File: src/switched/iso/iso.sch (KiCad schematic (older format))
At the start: 64 parts, among them IC1 NCP1252ADR2G, J1 Conn_01x02, J2 Conn_01x02, J3 Conn_01x02, J4 Conn_01x02, Q1 TSD5N50MR, Q2 TSD5N50MR, T1 Transformer_1P_1S, U1 NCP5106, U2 ORPC-817C, U3 TL431LP, U4 MC34072, U5 LM317_SOT-223

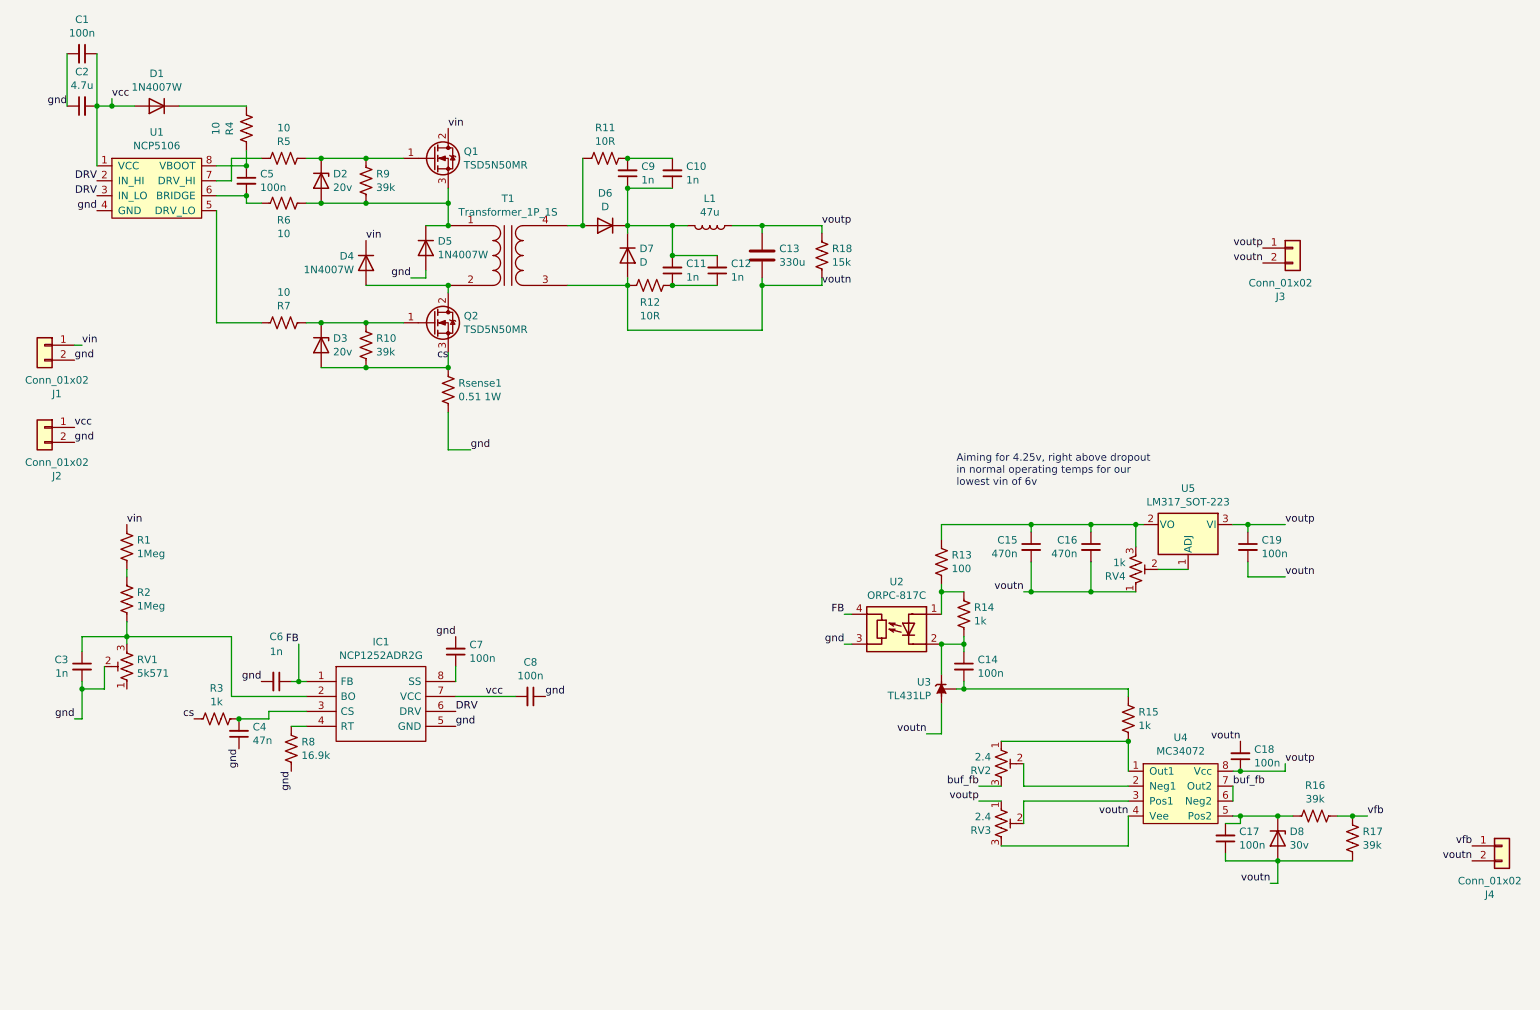
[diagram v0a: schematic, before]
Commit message: Midterm report
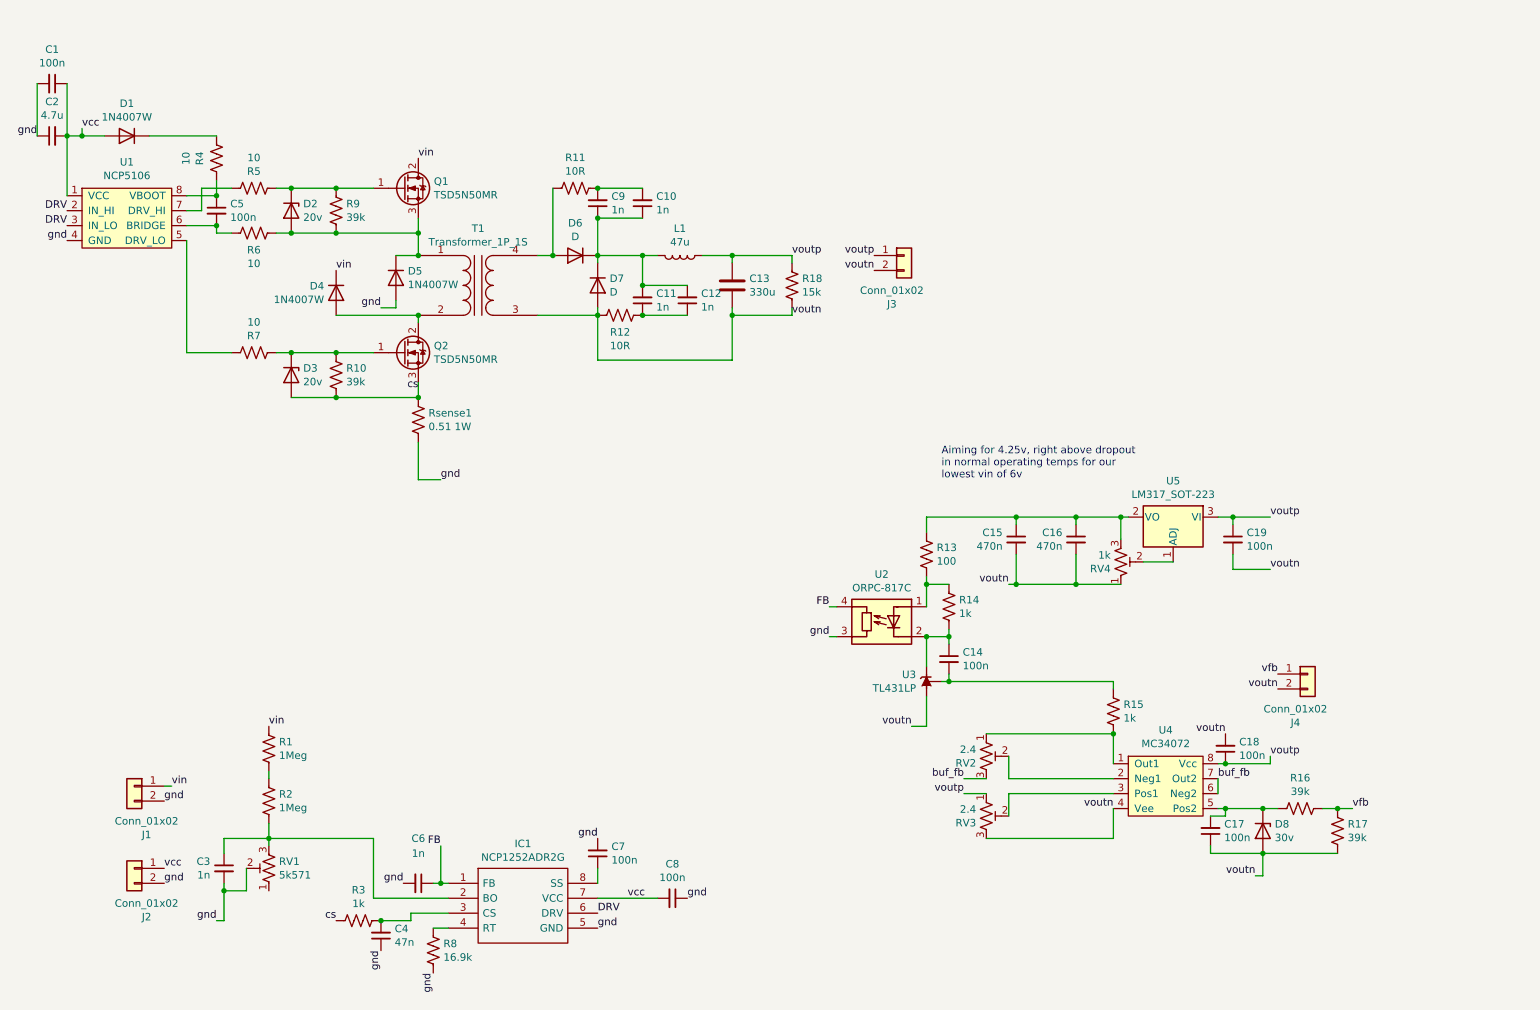
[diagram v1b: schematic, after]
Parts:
- C1, C14, C17, C18, C19, C5, C7, C8: Price (none) -> 0.0032
- C10, C11, C12, C3, C6, C9, R14, R15, R3: Price (none) -> 0.0031
- C13: Price (none) -> 0.1728
- C15, C16: Price (none) -> 0.0112
- C2: Price (none) -> 0.039
- C4: Price (none) -> 0.0036
- D1, D4, D5: Price (none) -> 0.0067
- D2, D3: Price (none) -> 0.0123
- D6, D7: Price (none) -> 0.0718
- D8: Price (none) -> 0.0173
- IC1: Price (none) -> 0.5338
- L1: Price (none) -> 0.6745
- Q1, Q2: Price (none) -> 0.1438
- R1, R2: Price (none) -> 0.0234
- R10, R16, R17, R18, R9: Price (none) -> 0.0071
- R11, R12: Price (none) -> 0.0081
- R13: Price (none) -> 0.0052
- R4, R5, R6, R7: Price (none) -> 0.0012
- R8: Price (none) -> 0.008
- RV1: Price (none) -> 0.0538
- RV2, RV3: Price (none) -> 0.055
- RV4: Price (none) -> 0.0536
- Rsense1: Price (none) -> 0.051
- T1: Price (none) -> 1.337
- U1: Price (none) -> 0.6077
- U2: Price (none) -> 0.0381
- U3: Price (none) -> 0.0228
- U4: Price (none) -> 0.1754
- U5: Price (none) -> 0.2599
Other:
- moved on the sheet: C1, C10, C11, C12, C13, C14, C15, C16, C17, C18, C19, C2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
